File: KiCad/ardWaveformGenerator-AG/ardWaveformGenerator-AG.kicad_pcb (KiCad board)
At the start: 2 copper layers, 80 x 66 mm, 47 parts, among them U1 Power in, U2 5-pin_4_buttons_+_common, U3 LM386, U4 Output, U5 5-pin_4_LED_header

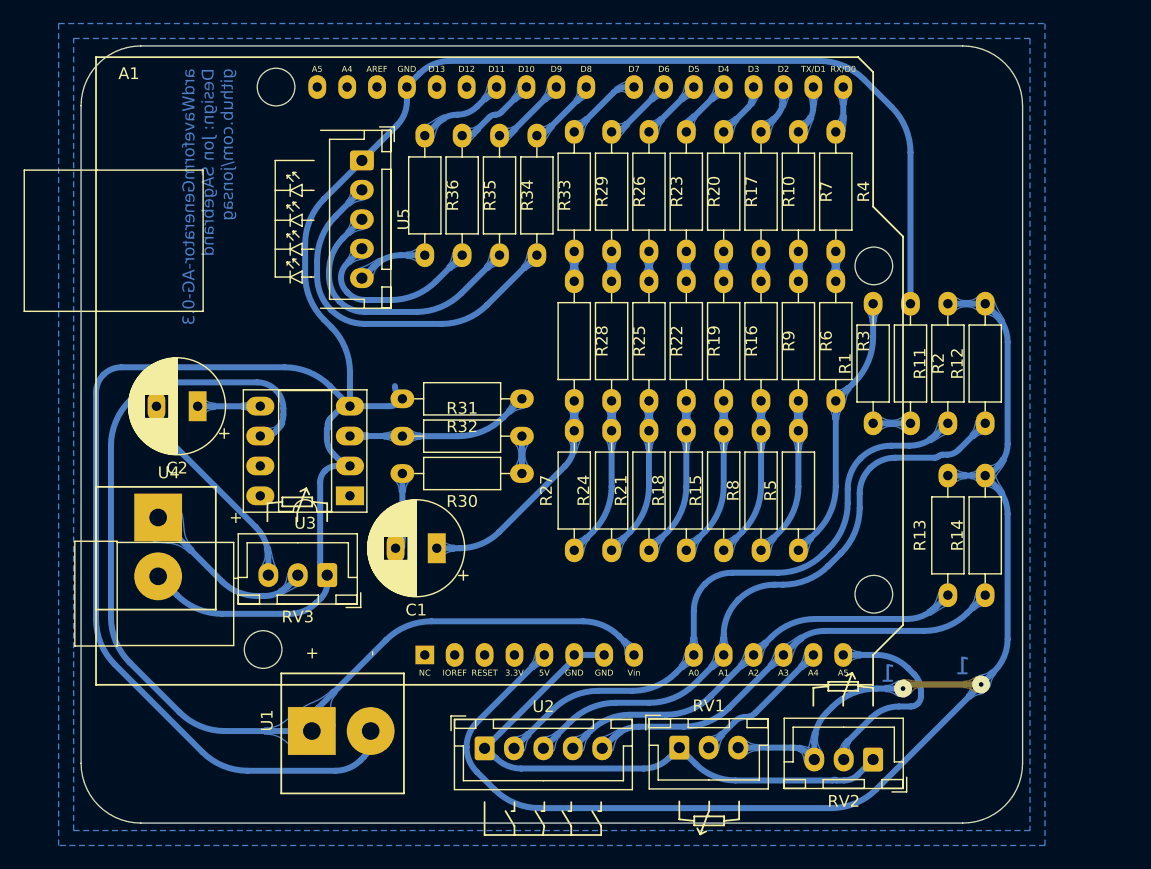
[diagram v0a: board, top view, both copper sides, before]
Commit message: VeroRoute and AG v0.4
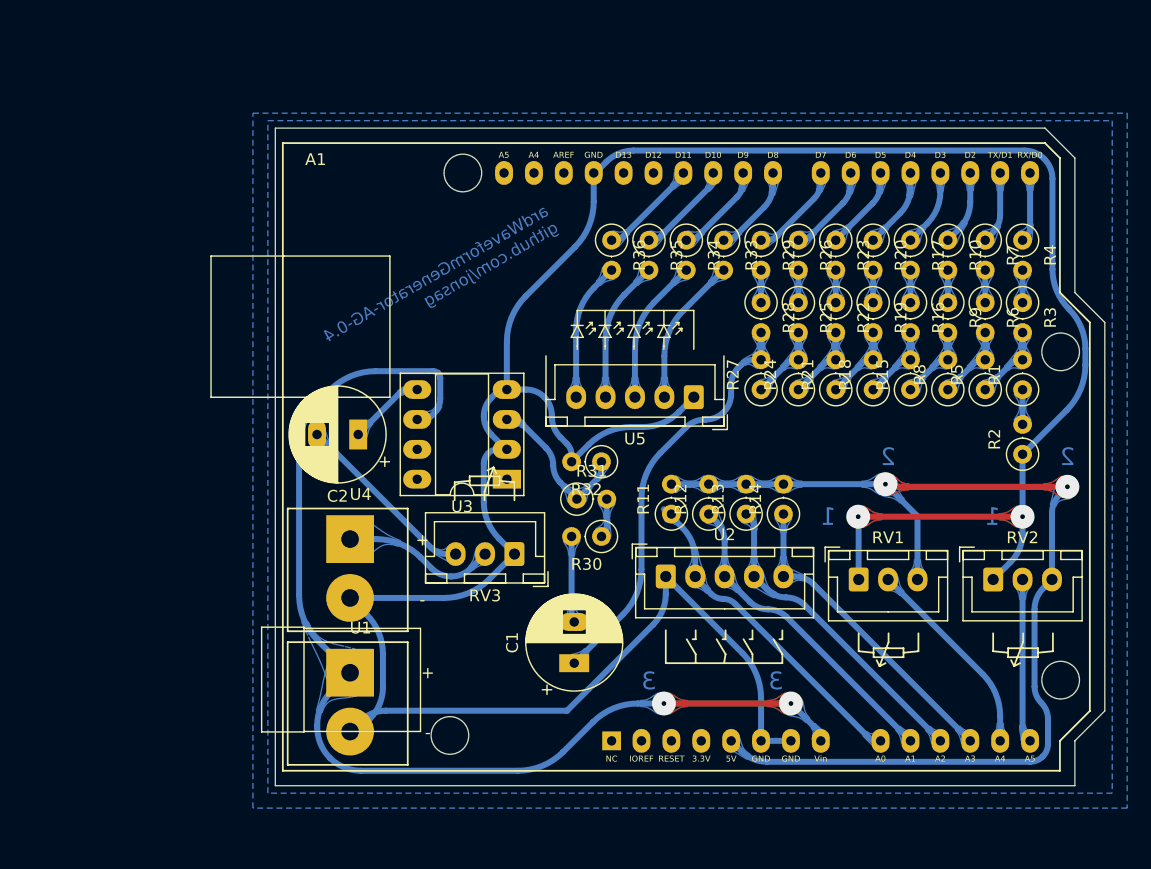
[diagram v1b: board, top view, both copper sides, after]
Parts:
- R1, R10, R11, R12, R13, R14, R15, R16, R17, R18, R19, R2, R20, R21, R22, R23, R24, R25, R26, R27, R28, R29, R3, R30, R31, R32, R33, R34, R35, R36, R4, R5, R6, R7, R8, R9: footprint My_Misc:R_Axial_DIN0207_L6.3mm_D2.5mm_P10.16mm_Horizontal_large -> My_Misc:R_Axial_DIN0207_L6.3mm_D2.5mm_P2.54mm_Vertical_large
- moved U5 34.6 mm to (165.1, 94.6), turned to 180 degrees
- moved R11 24.7 mm to (163.2, 104.5)
- moved R12 24.7 mm to (166.4, 104.5)
- moved U2 21.2 mm to (162.7, 109.9)
- moved R15 20.9 mm to (183.5, 94.0)
- moved R18 20.9 mm to (180.3, 94.0)
- moved R21 20.9 mm to (177.2, 94.0)
- moved R24 20.9 mm to (174.0, 94.0)
- moved R27 20.9 mm to (170.8, 94.0)
- moved R5 20.9 mm to (189.9, 94.0)
- moved R8 20.9 mm to (186.7, 94.0)
- moved RV1 20.9 mm to (179.1, 110.1)
- moved R13 18.5 mm to (169.5, 104.5)
- moved R14 18.5 mm to (172.7, 104.5)
- moved RV2 18.4 mm to (190.5, 110.1), turned to 0 degrees
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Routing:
- net +5V: track 126.4 -> 94.3 mm
- net A1: track 51.8 -> 27.1 mm
- net A0: track 52.2 -> 28.1 mm
- net Net-(D1-Pad2): track 31.8 -> 12.6 mm
- net GND: track 257.5 -> 238.6 mm, vias 0 -> 2
- net Net-(R1-Pad2): track 23.1 -> 6.36 mm
- net Net-(C1-Pad1): track 19.3 -> 35.2 mm
- net Net-(D2-Pad2): track 23.7 -> 12.3 mm
- net A3: track 37.0 -> 26.9 mm
- net A2: track 36.2 -> 26.9 mm
- net Net-(R21-Pad2): track 13.8 -> 6.36 mm
- net Net-(R15-Pad1): track 13.8 -> 6.36 mm
- net Net-(R24-Pad2): track 13.8 -> 6.36 mm
- net Net-(R5-Pad2): track 13.8 -> 6.36 mm
- net Net-(R18-Pad2): track 13.8 -> 6.36 mm
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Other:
- board size 80 x 66 mm -> 70.5 x 55.9 mm
- board text added: "${TITLE}-${REVISION} github.com/jonsag"
- board text added: "2"
- board text added: "3"
- board text removed: "${TITLE}-${REVISION} Design: Jon SAgebrand github.com/jonsag"
